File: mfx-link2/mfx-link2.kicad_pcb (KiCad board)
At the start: 2 copper layers, 50 x 50 mm, 52 parts, among them P1 CONN_01X04, P2 Gleisbox, P4 UART, P5 I2C, P6 CONN_02X03, P7 POTI, P8 IBT-2, Q1 BC817-40, T1 53040C, U1 6N137, U2 7805, U3 LM393, U4 78L05, U5 PIC16F1709

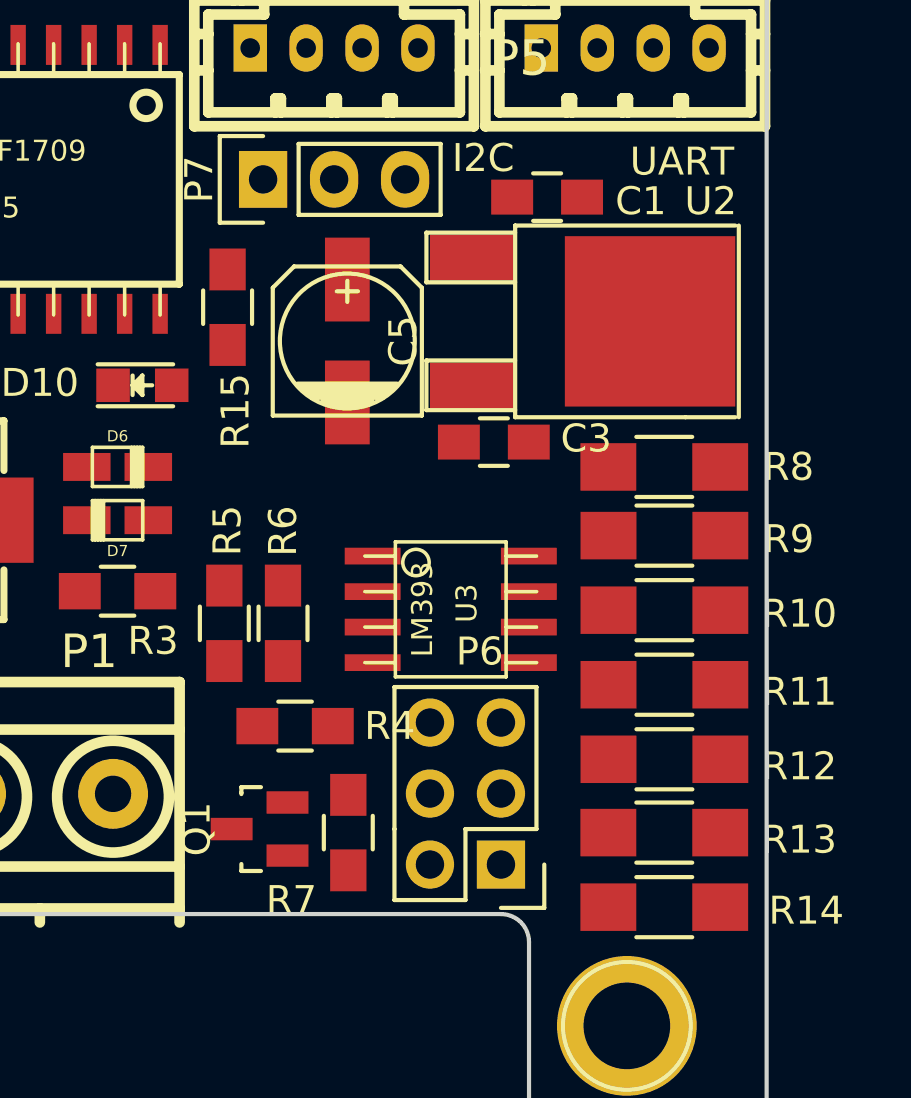
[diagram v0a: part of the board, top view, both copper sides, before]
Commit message: wip
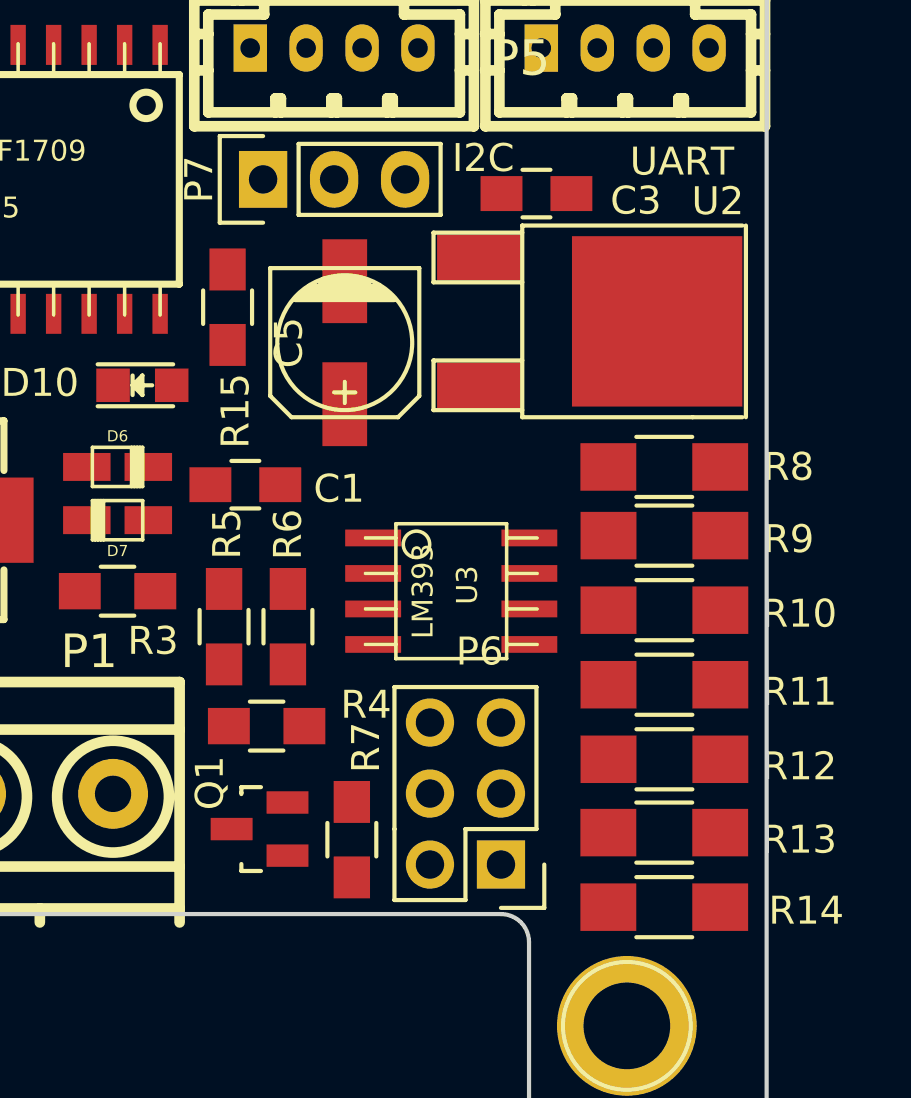
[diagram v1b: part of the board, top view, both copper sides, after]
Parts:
- moved C1 14.9 mm to (149.4, 104.1)
- moved C3 9.02 mm to (159.8, 93.7), turned to 0 degrees
- moved R4 1.02 mm to (150.1, 112.8)
- moved U3 0.65 mm to (156.7, 108.0)
- moved R7 0.28 mm to (153.2, 116.8)
- moved U2 0.25 mm to (157.7, 98.3)
- moved R6 0.21 mm to (150.9, 109.2)
- moved R5 0.12 mm to (148.6, 109.2)
- moved C5 0.11 mm to (152.9, 99.1), turned to 270 degrees
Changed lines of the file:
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@@
   )
   (module Capacitors_SMD:C_0805_HandSoldering (layer F.Cu)
-    (at 160.147 93.853)
+    (at 149.352 104.14)
     (descr "Capacitor SMD 0805, hand soldering")
     (tags "capacitor 0805")
@@
   )
   (module Capacitors_SMD:C_0805_HandSoldering (layer F.Cu)
-    (at 158.242 102.616 180)
+    (at 159.766 93.726)
     (descr "Capacitor SMD 0805, hand soldering")
     (tags "capacitor 0805")
     (attr smd)
-    (fp_text reference C3 (at -3.302 0.127 180) (layer F.SilkS)
-      (effects (font (size 1 1) (thickness 0.15)))
-    )
-    (fp_text value 100nF (at 0.0508 0.2794 180) (layer F.Fab)
+    (fp_text reference C3 (at 3.556 0.254) (layer F.SilkS)
+      (effects (font (size 1 1) (thickness 0.15)))
+    )
+    (fp_text value 100nF (at 0.0508 0.2794) (layer F.Fab)
       (effects (font (size 1 1) (thickness 0.15)))
     )
@@
     (fp_line (start 0.5 -0.85) (end -0.5 -0.85) (layer F.SilkS) (width 0.15))
     (fp_line (start -0.5 0.85) (end 0.5 0.85) (layer F.SilkS) (width 0.15))
-    (pad 1 smd rect (at -1.25 0 180) (size 1.5 1.25) (layers F.Cu F.Paste F.Mask)
+    (pad 1 smd rect (at -1.25 0) (size 1.5 1.25) (layers F.Cu F.Paste F.Mask)
       (net 41 /18V+))
-    (pad 2 smd rect (at 1.25 0 180) (size 1.5 1.25) (layers F.Cu F.Paste F.Mask)
+    (pad 2 smd rect (at 1.25 0) (size 1.5 1.25) (layers F.Cu F.Paste F.Mask)
       (net 4 GND))
     (model Capacitors_SMD.3dshapes/C_0805_HandSoldering.wrl
@@
     (tags SOT-23)
     (attr smd)
-    (fp_text reference Q1 (at 0 -2.25 90) (layer F.SilkS)
+    (fp_text reference Q1 (at 1.651 -1.778 90) (layer F.SilkS)
       (effects (font (size 1 1) (thickness 0.15)))
     )
@@
   )
   (module Resistors_SMD:R_0805_HandSoldering (layer F.Cu)
-    (at 151.13 112.776)
+    (at 150.114 112.776)
     (descr "Resistor SMD 0805, hand soldering")
     (tags "resistor 0805")
     (attr smd)
-    (fp_text reference R4 (at 3.39 -0.005) (layer F.SilkS)
+    (fp_text reference R4 (at 3.556 -0.762) (layer F.SilkS)
       (effects (font (size 1 1) (thickness 0.15)))
     )
@@
   )
   (module Resistors_SMD:R_0805_HandSoldering (layer F.Cu)
-    (at 148.6 109.1 270)
+    (at 148.59 109.22 270)
     (descr "Resistor SMD 0805, hand soldering")
     (tags "resistor 0805")
@@
   )
   (module Resistors_SMD:R_0805_HandSoldering (layer F.Cu)
-    (at 150.7 109.1 90)
+    (at 150.876 109.22 90)
     (descr "Resistor SMD 0805, hand soldering")
     (tags "resistor 0805")
@@
   )
   (module Resistors_SMD:R_0805_HandSoldering (layer F.Cu)
-    (at 153.035 116.586 270)
+    (at 153.162 116.84 270)
     (descr "Resistor SMD 0805, hand soldering")
     (tags "resistor 0805")
     (attr smd)
-    (fp_text reference R7 (at 2.414 2.035 360) (layer F.SilkS)
+    (fp_text reference R7 (at -3.302 -0.508 450) (layer F.SilkS)
       (effects (font (size 1 1) (thickness 0.15)))
     )
@@
   )
   (module 78xx:TO-252-2Lead (layer F.Cu)
-    (at 157.48 98.298 270)
+    (at 157.734 98.298 270)
     (descr "DPAK / TO-252 2-lead smd package")
     (tags "dpak TO-252")
@@
   )
   (module w_smd_dil:so-8 (layer F.Cu)
-    (at 156.7 108.6 270)
+    (at 156.718 107.95 270)
     (descr SO-8)
     (fp_text reference U3 (at -0.2186 -0.5704 270) (layer F.SilkS)
@@
   )
   (module Capacitors_SMD:c_elec_5x5.3 (layer F.Cu)
-    (at 153 99 90)
+    (at 152.908 99.06 270)
     (descr "SMT capacitor, aluminium electrolytic, 5x5.3")
     (attr smd)
-    (fp_text reference C5 (at 0 2 90) (layer F.SilkS)
-      (effects (font (size 1 1) (thickness 0.15)))
-    )
-    (fp_text value 47uF (at 0 3.81 90) (layer F.Fab)
+    (fp_text reference C5 (at 0 2 270) (layer F.SilkS)
+      (effects (font (size 1 1) (thickness 0.15)))
+    )
+    (fp_text value 47uF (at 0 3.81 270) (layer F.Fab)
       (effects (font (size 1 1) (thickness 0.15)))
     )
@@
     (fp_line (start 1.778 -0.381) (end 1.778 0.381) (layer F.SilkS) (width 0.15))
     (fp_circle (center 0 0) (end -2.413 0) (layer F.SilkS) (width 0.15))
-    (pad 1 smd rect (at 2.19964 0 90) (size 2.99974 1.6002) (layers F.Cu F.Paste F.Mask)
+    (pad 1 smd rect (at 2.19964 0 270) (size 2.99974 1.6002) (layers F.Cu F.Paste F.Mask)
       (net 6 VCC))
-    (pad 2 smd rect (at -2.19964 0 90) (size 2.99974 1.6002) (layers F.Cu F.Paste F.Mask)
+    (pad 2 smd rect (at -2.19964 0 270) (size 2.99974 1.6002) (layers F.Cu F.Paste F.Mask)
       (net 4 GND))
     (model Capacitors_SMD.3dshapes/c_elec_5x5.3.wrl
